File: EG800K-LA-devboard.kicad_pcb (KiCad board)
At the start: 4 copper layers, 35 x 36.5 mm, 52 parts, among them J1 U.FL-R-SMT_10_, J2 MICROQTJ, J4 Conn_01x11_Pin, Q1 DTC143ZUAT106, Q2 DTC143ZUAT106, Q3 AO3415, Q4 DTC143ZUAT106, Q5 DTC143ZUAT106, U1 EG800KEULC-I03-SNNSA, U2 TP4057

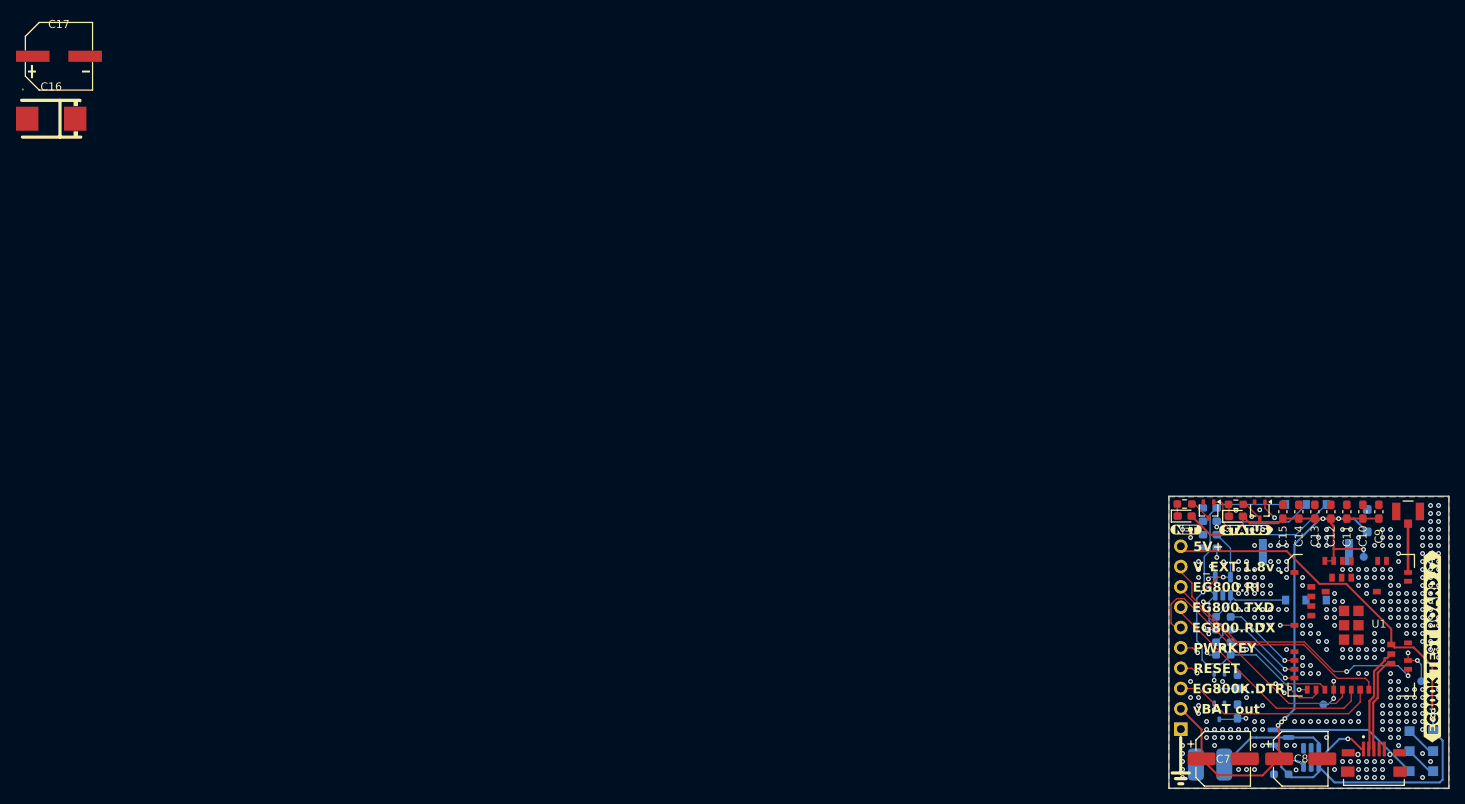
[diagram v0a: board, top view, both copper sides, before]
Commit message: carga final
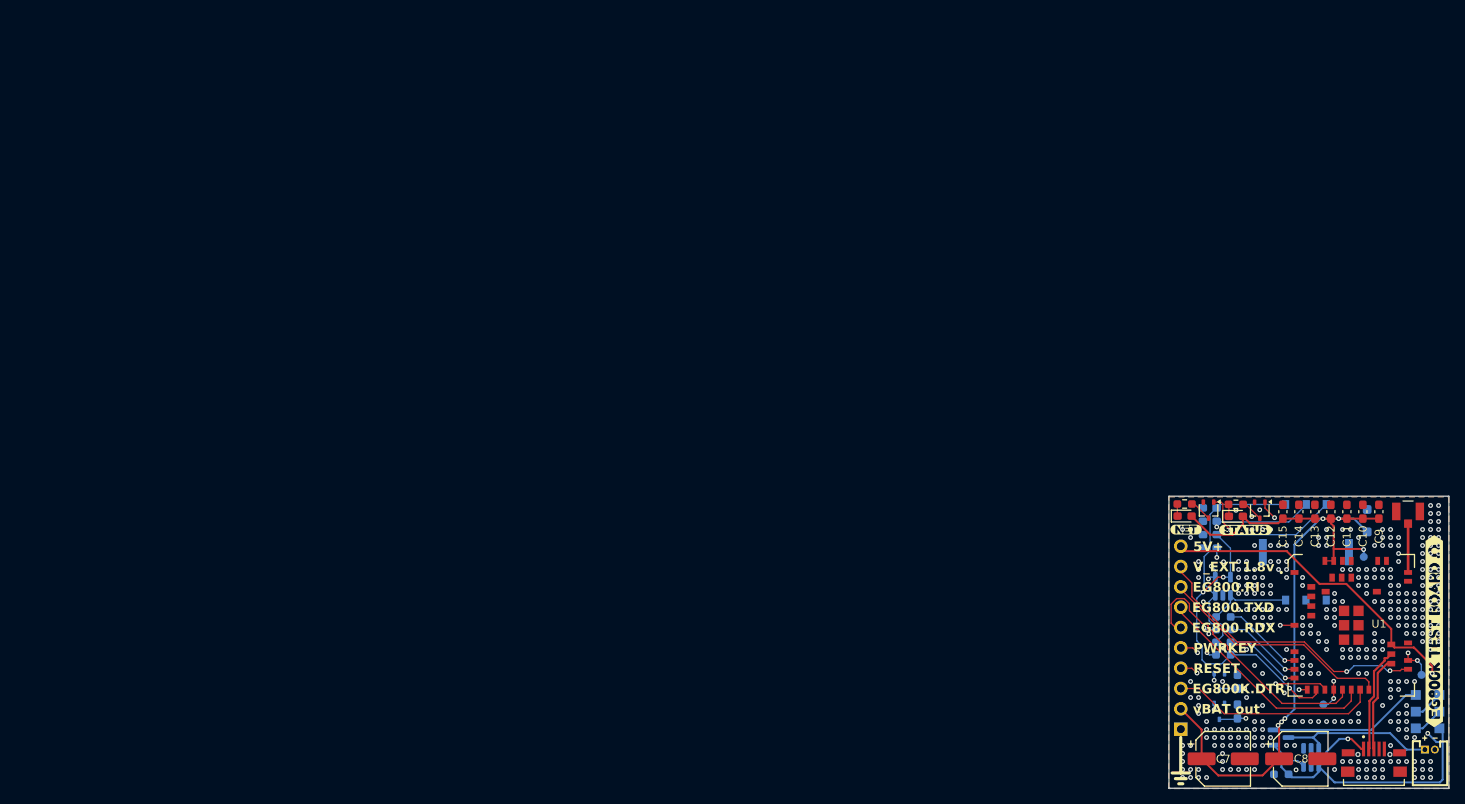
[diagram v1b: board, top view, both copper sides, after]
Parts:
- removed BAT+1: BAT+, Connector_Wire:SolderWirePad_1x01_SMD_2x4mm
- removed BAT-1: BAT-, Connector_Wire:SolderWirePad_1x01_SMD_2x4mm
- removed C16: TAJD337K010RNJ, EasyEDA:CASE-D_7343
- removed C17: VT1A102M0810, EasyEDA:CAP-SMD_BD8.0-L8.3-W8.3-FD
- added CN1: 530480210, EasyEDA:CONN-TH_530480210, F.Cu at (176.7, 91.0)
- moved D4 9.55 mm to (176.4, 84.1)
- moved D3 4.99 mm to (176.4, 86.2)
- moved kibuzzard-6A1B8E1D 1.91 mm to (177.3, 76.2)
- moved D2 0.85 mm to (176.4, 88.3)
- moved REF** 0.79 mm to (175.7, 81.6)
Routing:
- net +4.2V: track 14.2 -> 19.8 mm
- net +5V: track 88.6 -> 90.3 mm, vias 4 -> 3
- net /EG800K.UART1_RXD: track 32.4 -> 33.5 mm
- net /EG800K.VDD_ETX: track 36.9 -> 35.9 mm
- net /EG800K.STATUS: track 31.1 -> 30.4 mm
- net GND: vias 327 -> 330
